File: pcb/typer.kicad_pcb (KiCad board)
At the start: 2 copper layers, 182.8 x 158.9 mm, 46 parts, among them J2 3.5mm, SW0:0 SW0:0, SW0:1 SW0:1, SW0:2 SW0:2, SW0:3 SW0:3, SW0:4 SW0:4, SW1:0 SW1:0, SW1:1 SW1:1, SW1:2 SW1:2, SW1:3 SW1:3, SW1:4 SW1:4, SW2:0 SW2:0, SW2:1 SW2:1, SW2:2 SW2:2, SW2:3 SW2:3, SW2:4 SW2:4, SW3:0 SW3:0, SW3:1 SW3:1, SW3:2 SW3:2, SW3:3 SW3:3, SW3:4 SW3:4, SW4:0 SW4:0, SW4:1 SW4:1, SW4:2 SW4:2, SW4:3 SW4:3, SW4:4 SW4:4, SW5:0 SW5:0, SW5:1 SW5:1, SW5:2 SW5:2, SW5:3 SW5:3, SW5:4 SW5:4, SW6:0 SW6:0, SW6:1 SW6:1, SW6:2 SW6:2, SW6:3 SW6:3, SW6:4 SW6:4, SW7:2 SW7:2, SW7:3 SW7:3, SW7:4 SW7:4, U1 rp2040-zero

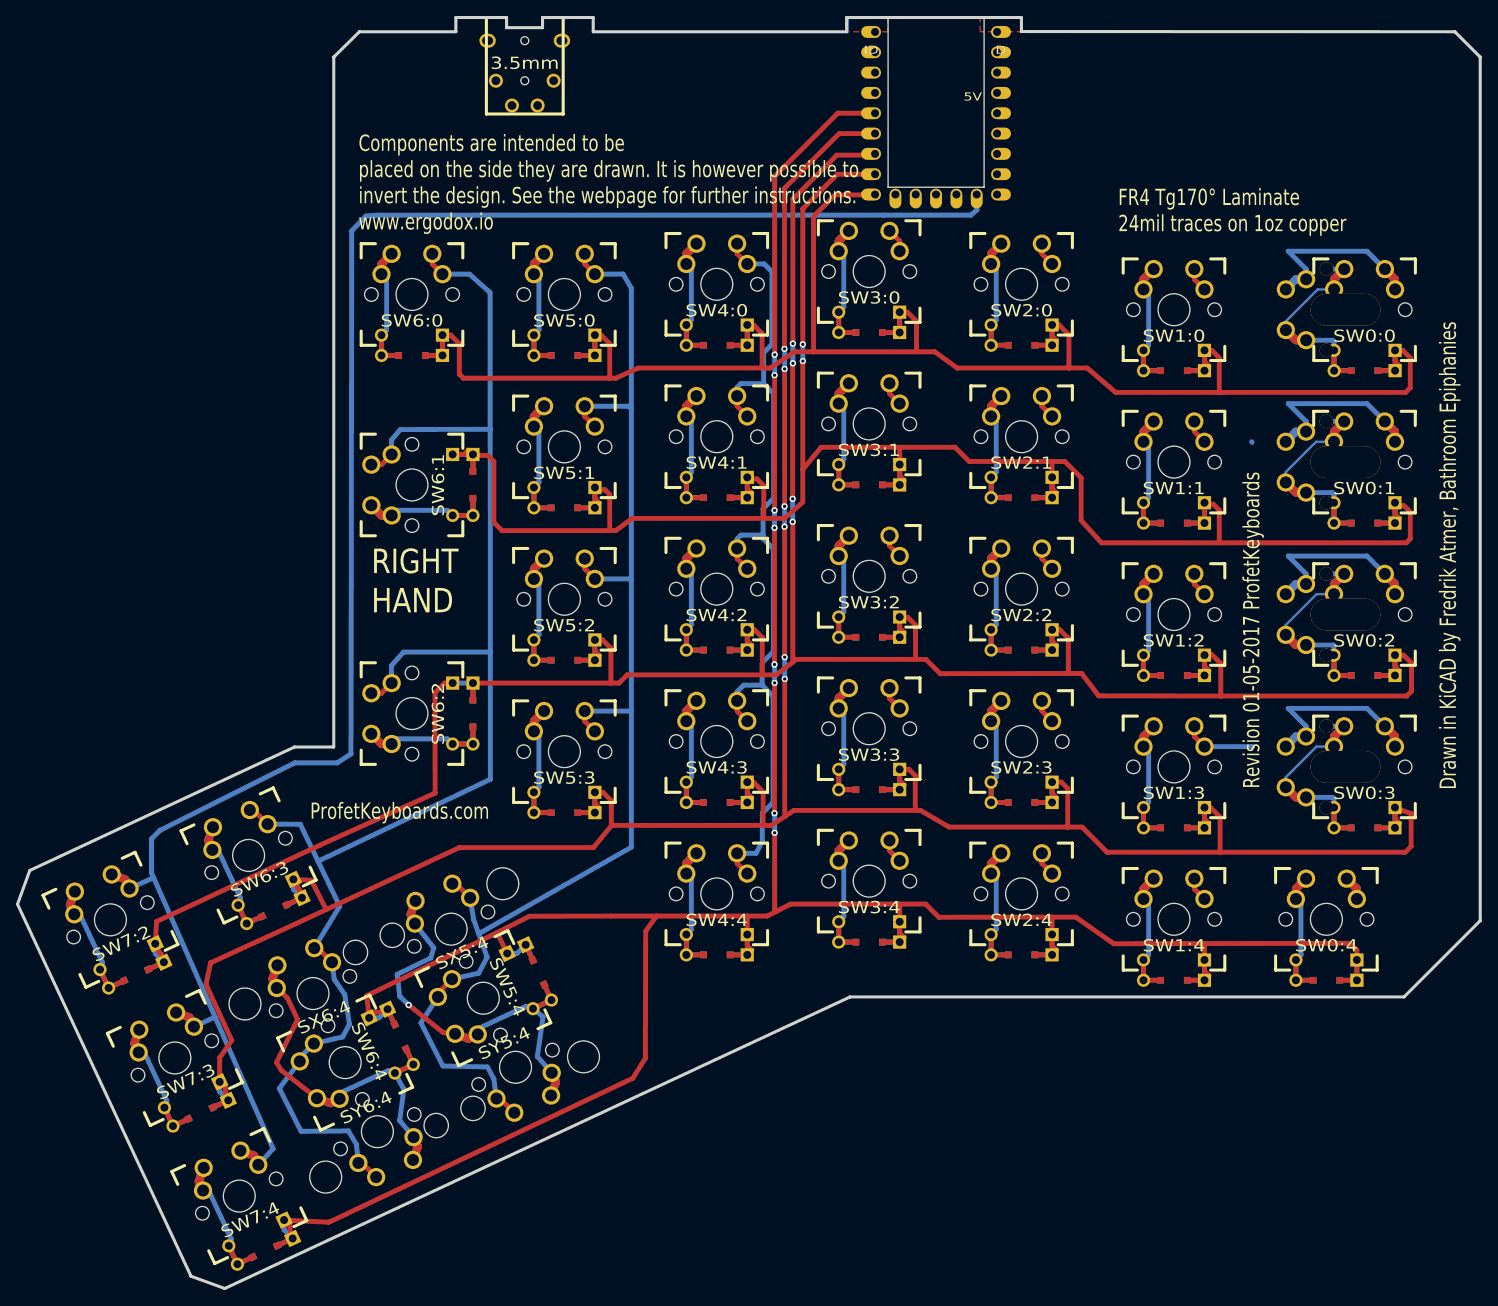
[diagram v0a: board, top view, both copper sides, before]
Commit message: added holes
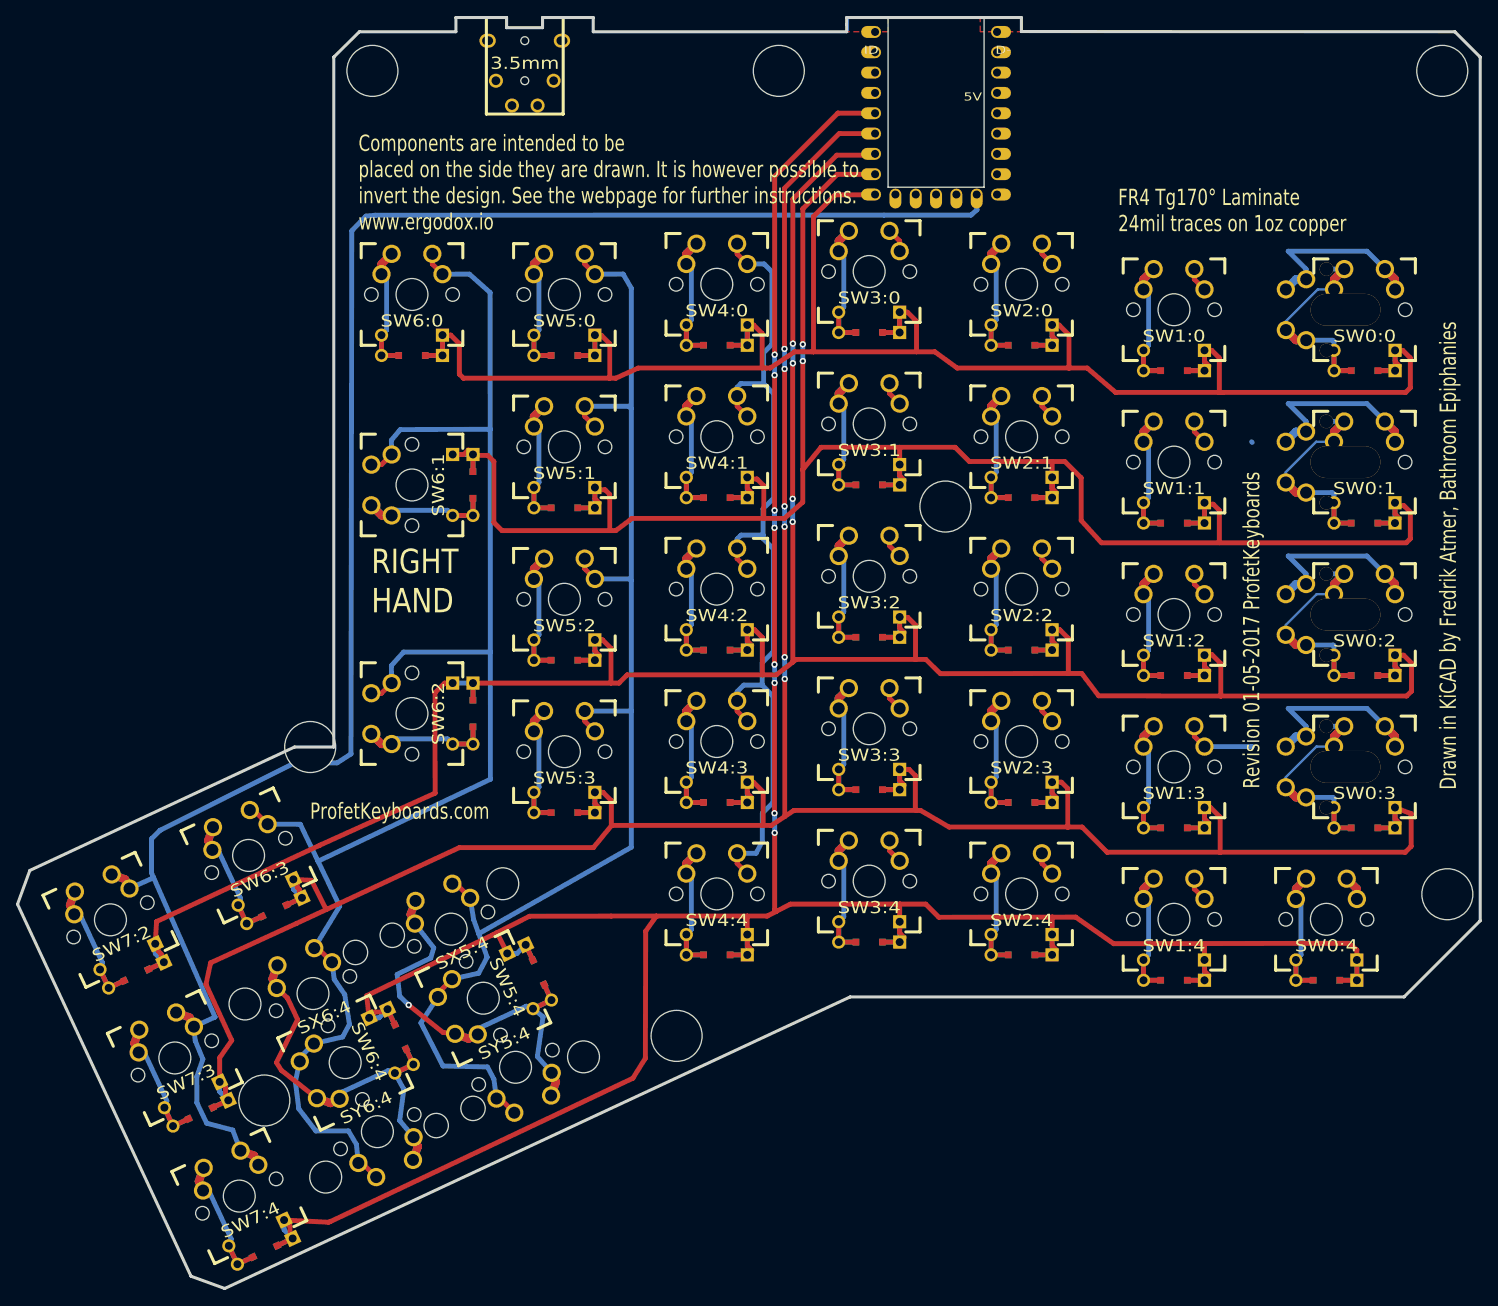
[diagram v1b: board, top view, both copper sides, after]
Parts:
- added H99: MECHANICAL, ErgoDOXmech, F.Cu at (50.8, 177.8)
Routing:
- net COLUMN6: track 198.8 -> 196.2 mm
- net COLUMN7: track 243.5 -> 241.6 mm
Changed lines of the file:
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@@
     (pad "99" smd rect locked (at 1.6637 7.62 115) (size 0.8382 0.8382) (layers "B.Cu" "B.Paste" "B.Mask"))
   )
+  (footprint "ErgoDOXmech" (layer "F.Cu")
+    (at 50.8306 177.8142)
+    (attr through_hole)
+    (fp_text reference "H99" (at 0 0 90) (layer "F.SilkS") hide
+        (effects (font (size 0.762 0.762) (thickness 0.1524)))
+    )
+    (fp_text value "MECHANICAL" (at 0 0 90) (layer "F.SilkS") hide
+        (effects (font (size 0.762 0.762) (thickness 0.1524)))
+    )
+    (pad "" np_thru_hole circle (at 3.0988 -11.9634) (size 6.3754 6.3754) (drill 6.3754) (layers "F&B.Cu" "*.Mask")
+      (solder_mask_margin -0.254) (zone_connect 2))
+    (pad "" np_thru_hole circle locked (at 8.834 -56.1482) (size 6.3754 6.3754) (drill 6.3754) (layers "F&B.Cu" "*.Mask")
+      (solder_mask_margin -0.254) (zone_connect 2))
+    (pad "" np_thru_hole circle (at 16.6116 -140.6652) (size 6.3754 6.3754) (drill 6.3754) (layers "F&B.Cu" "*.Mask")
+      (solder_mask_margin -0.254) (zone_connect 2))
+    (pad "" np_thru_hole circle (at 54.6354 -20.0406) (size 6.3754 6.3754) (drill 6.3754) (layers "F&B.Cu" "*.Mask")
+      (solder_mask_margin -0.254) (zone_connect 2))
+    (pad "" np_thru_hole circle (at 67.4116 -140.6652) (size 6.3754 6.3754) (drill 6.3754) (layers "F&B.Cu" "*.Mask")
+      (solder_mask_margin -0.254) (zone_connect 2))
+    (pad "" np_thru_hole circle (at 88.2396 -86.2076) (size 6.3754 6.3754) (drill 6.3754) (layers "F&B.Cu" "*.Mask")
+      (solder_mask_margin -0.254) (zone_connect 2))
+    (pad "" np_thru_hole circle (at 150.3426 -140.6652) (size 6.3754 6.3754) (drill 6.3754) (layers "F&B.Cu" "*.Mask")
+      (solder_mask_margin -0.254) (zone_connect 2))
+    (pad "" np_thru_hole circle (at 150.9776 -37.7444) (size 6.3754 6.3754) (drill 6.3754) (layers "F&B.Cu" "*.Mask")
+      (solder_mask_margin -0.254) (zone_connect 2))
+  )
   (footprint "Library:MX_FLIP_DIODE" locked (layer "F.Cu")
     (at 51.9633 135.219 25)
@@
     (effects (font (size 2.032 1.524) (thickness 0.3048)) (justify left))
   )
+  (dimension (type aligned) (layer "B.Cu")
+    (pts (xy 68.0222 32.429) (xy 68.0222 33.679))
+    (height 11.65)
+    (gr_text "1.2500 mm" (at 54.5722 33.054 90) (layer "B.Cu")
+      (effects (font (size 1.5 1.5) (thickness 0.3)))
+    )
+    (format (prefix "") (suffix "") (units 3) (units_format 1) (precision 4))
+    (style (thickness 0.2) (arrow_length 1.27) (text_position_mode 0) (extension_height 0.58642) (extension_offset 0.5) keep_text_aligned)
+  )
+  (dimension (type aligned) (layer "B.Cu")
+    (pts (xy 63.9822 37.339) (xy 62.8122 37.339))
+    (height 14.36)
+    (gr_text "1.1700 mm" (at 63.3972 21.179) (layer "B.Cu")
+      (effects (font (size 1.5 1.5) (thickness 0.3)))
+    )
+    (format (prefix "") (suffix "") (units 3) (units_format 1) (precision 4))
+    (style (thickness 0.2) (arrow_length 1.27) (text_position_mode 0) (extension_height 0.58642) (extension_offset 0.5) keep_text_aligned)
+  )
   (segment (start 195.2625 63.1952) (end 195.2625 64.4652) (width 1.016) (layer "F.Cu") (net 7))
   (segment (start 195.2625 82.24266) (end 195.2625 83.51266) (width 1.016) (layer "F.Cu") (net 7))
@@
   (segment (start 67.31 86.3702) (end 68.58 86.3702) (width 0.6096) (layer "F.Cu") (net 44))
   (segment (start 52.118421 129.541506) (end 52.577585 129.541506) (width 0.6096) (layer "F.Cu") (net 44))
-  (segment (start 58.361006 160.961879) (end 55.8022 164.349) (width 0.6096) (layer "B.Cu") (net 44))
   (segment (start 58.361006 160.961879) (end 58.361006 160.502715) (width 0.6096) (layer "B.Cu") (net 44))
   (segment (start 71.3322 109.799) (end 82.181746 109.799) (width 0.6096) (layer "B.Cu") (net 44))
@@
   (segment (start 82.1522 64.859) (end 82.163436 81.949) (width 0.6096) (layer "B.Cu") (net 44))
   (segment (start 63.3522 141.569) (end 60.170221 146.806506) (width 0.6096) (layer "B.Cu") (net 44))
-  (segment (start 64.4522 169.659) (end 65.4422 171.339) (width 0.6096) (layer "B.Cu") (net 44))
   (segment (start 70.9222 81.989) (end 82.163436 81.949) (width 0.6096) (layer "B.Cu") (net 44))
   (segment (start 60.646871 135.944329) (end 63.3522 141.569) (width 0.6096) (layer "B.Cu") (net 44))
   (segment (start 69.8122 111.499) (end 71.3322 109.799) (width 0.6096) (layer "B.Cu") (net 44))
+  (segment (start 65.4422 171.339) (end 65.684818 173.660197) (width 0.6096) (layer "B.Cu") (net 44))
   (segment (start 64.5722 156.319) (end 63.7222 157.909) (width 0.6096) (layer "B.Cu") (net 44))
+  (segment (start 57.8122 163.479) (end 58.2422 166.889) (width 0.6096) (layer "B.Cu") (net 44))
   (segment (start 69.8122 83.319) (end 70.9222 81.989) (width 0.6096) (layer "B.Cu") (net 44))
   (segment (start 82.1922 125.699) (end 60.646871 135.944329) (width 0.6096) (layer "B.Cu") (net 44))
-  (segment (start 55.8022 164.349) (end 58.5322 169.699) (width 0.6096) (layer "B.Cu") (net 44))
   (segment (start 58.4222 131.319) (end 60.646871 135.944329) (width 0.6096) (layer "B.Cu") (net 44))
+  (segment (start 64.4522 169.659) (end 65.4422 171.339) (width 0.6096) (layer "B.Cu") (net 44))
+  (segment (start 58.361006 160.961879) (end 57.8122 163.479) (width 0.6096) (layer "B.Cu") (net 44))
   (segment (start 69.85 85.1002) (end 69.8122 83.319) (width 0.6096) (layer "B.Cu") (net 44))
   (segment (start 54.342882 131.306803) (end 58.4222 131.319) (width 0.6096) (layer "B.Cu") (net 44))
+  (segment (start 58.2422 166.889) (end 60.3722 169.659) (width 0.6096) (layer "B.Cu") (net 44))
   (segment (start 76.2 62.5602) (end 76.5302 62.8904) (width 0.6096) (layer "B.Cu") (net 44))
   (segment (start 58.361006 160.502715) (end 60.126303 158.737418) (width 0.6096) (layer "B.Cu") (net 44))
   (segment (start 62.6722 150.709) (end 63.9822 152.599) (width 0.6096) (layer "B.Cu") (net 44))
   (segment (start 82.163436 81.949) (end 82.181746 109.799) (width 0.6096) (layer "B.Cu") (net 44))
-  (segment (start 58.5322 169.699) (end 64.4522 169.659) (width 0.6096) (layer "B.Cu") (net 44))
   (segment (start 63.9822 152.599) (end 64.5722 156.319) (width 0.6096) (layer "B.Cu") (net 44))
   (segment (start 63.7222 157.909) (end 60.126303 158.737418) (width 0.6096) (layer "B.Cu") (net 44))
   (segment (start 79.5722 62.559) (end 82.1522 64.859) (width 0.6096) (layer "B.Cu") (net 44))
   (segment (start 76.2 62.5602) (end 79.5722 62.559) (width 0.6096) (layer "B.Cu") (net 44))
-  (segment (start 65.4422 171.339) (end 65.684818 173.660197) (width 0.6096) (layer "B.Cu") (net 44))
   (segment (start 69.85 113.675) (end 69.8122 111.499) (width 0.6096) (layer "B.Cu") (net 44))
+  (segment (start 60.3722 169.659) (end 64.4522 169.659) (width 0.6096) (layer "B.Cu") (net 44))
   (segment (start 62.394682 148.571803) (end 62.6722 150.709) (width 0.6096) (layer "B.Cu") (net 44))
   (segment (start 68.58 61.2902) (end 68.58 62.5602) (width 1.016) (layer "F.Cu") (net 45))
@@
   (segment (start 142.2722 55.179) (end 131.3922 55.179) (width 0.6096) (layer "B.Cu") (net 50))
   (segment (start 131.3922 55.179) (end 67.8122 55.189) (width 0.6096) (layer "B.Cu") (net 50))
-  (segment (start 55.0322 171.889) (end 47.776334 155.424866) (width 0.6096) (layer "B.Cu") (net 50))
+  (segment (start 45.4922 162.879) (end 45.5022 166.129) (width 0.6096) (layer "B.Cu") (net 50))
   (segment (start 40.9222 132.069) (end 57.7322 123.649) (width 0.6096) (layer "B.Cu") (net 50))
+  (segment (start 46.7222 168.689) (end 49.9822 169.549) (width 0.6096) (layer "B.Cu") (net 50))
   (segment (start 64.7622 122.539) (end 64.8622 57.139) (width 0.6096) (layer "B.Cu") (net 50))
   (segment (start 63.0322 123.649) (end 64.7622 122.539) (width 0.6096) (layer "B.Cu") (net 50))
@@
   (segment (start 37.078482 139.356803) (end 40.095271 137.995929) (width 0.6096) (layer "B.Cu") (net 50))
   (segment (start 40.9022 132.069) (end 40.9222 132.069) (width 0.6096) (layer "B.Cu") (net 50))
-  (segment (start 53.179582 173.887803) (end 55.0322 171.889) (width 0.6096) (layer "B.Cu") (net 50))
+  (segment (start 45.2922 158.379) (end 46.2522 160.689) (width 0.6096) (layer "B.Cu") (net 50))
+  (segment (start 46.2522 160.689) (end 45.4922 162.879) (width 0.6096) (layer "B.Cu") (net 50))
+  (segment (start 49.9822 169.549) (end 50.955121 172.122506) (width 0.6096) (layer "B.Cu") (net 50))
+  (segment (start 45.5022 166.129) (end 46.7222 168.689) (width 0.6096) (layer "B.Cu") (net 50))
   (segment (start 34.85388 137.5918) (end 36.54044 138.20648) (width 1.016) (layer "B.Cu") (net 50))
   (segment (start 47.776334 155.424866) (end 40.095271 137.995929) (width 0.6096) (layer "B.Cu") (net 50))
+  (segment (start 45.127782 156.620803) (end 45.2922 158.379) (width 0.6096) (layer "B.Cu") (net 50))
   (segment (start 57.7322 123.649) (end 63.0322 123.649) (width 0.6096) (layer "B.Cu") (net 50))
   (segment (start 143.0122 54.519) (end 142.2722 55.179) (width 0.6096) (layer "B.Cu") (net 50))
